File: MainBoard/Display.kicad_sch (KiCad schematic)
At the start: 2 parts, among them CN1 HC-FPC-05-09-22RLTAG, Q2 MMBT2222ALT1G

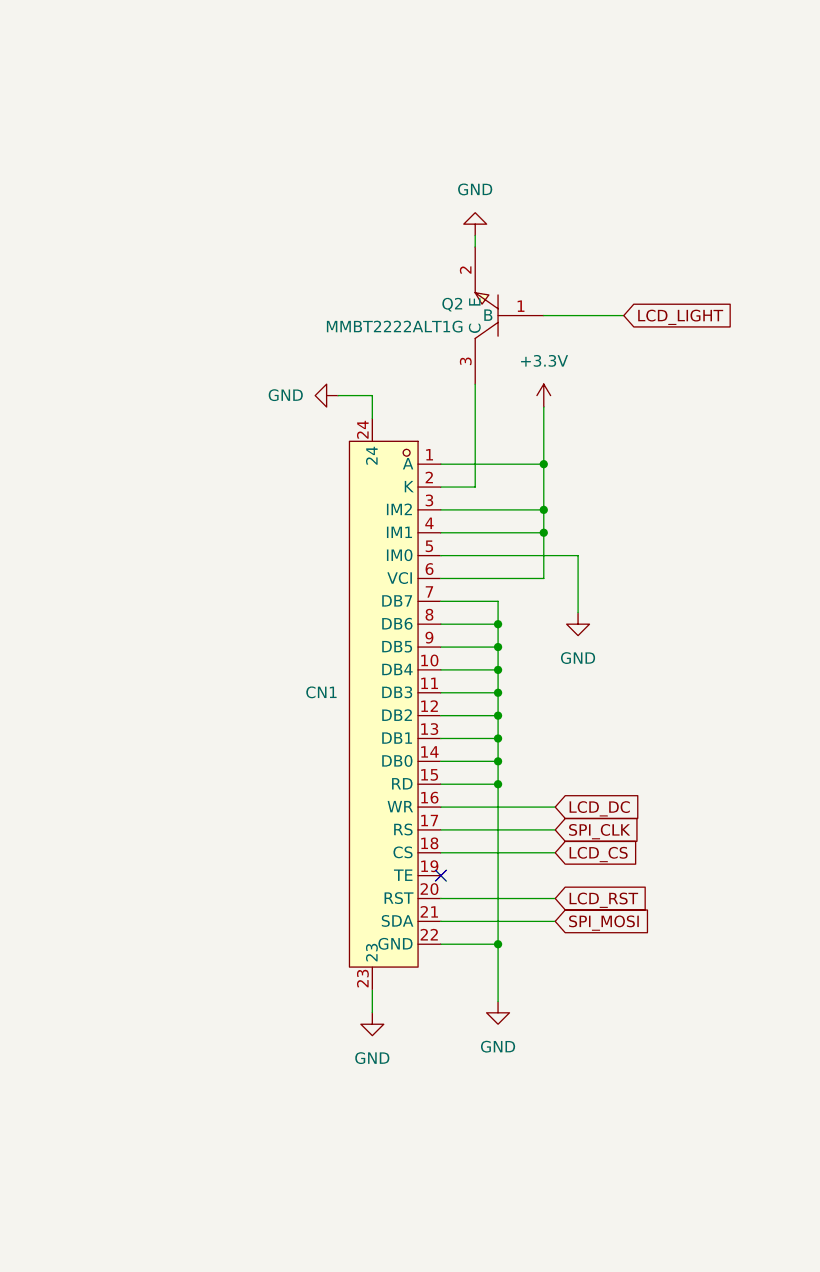
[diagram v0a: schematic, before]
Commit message: layout and starting routing
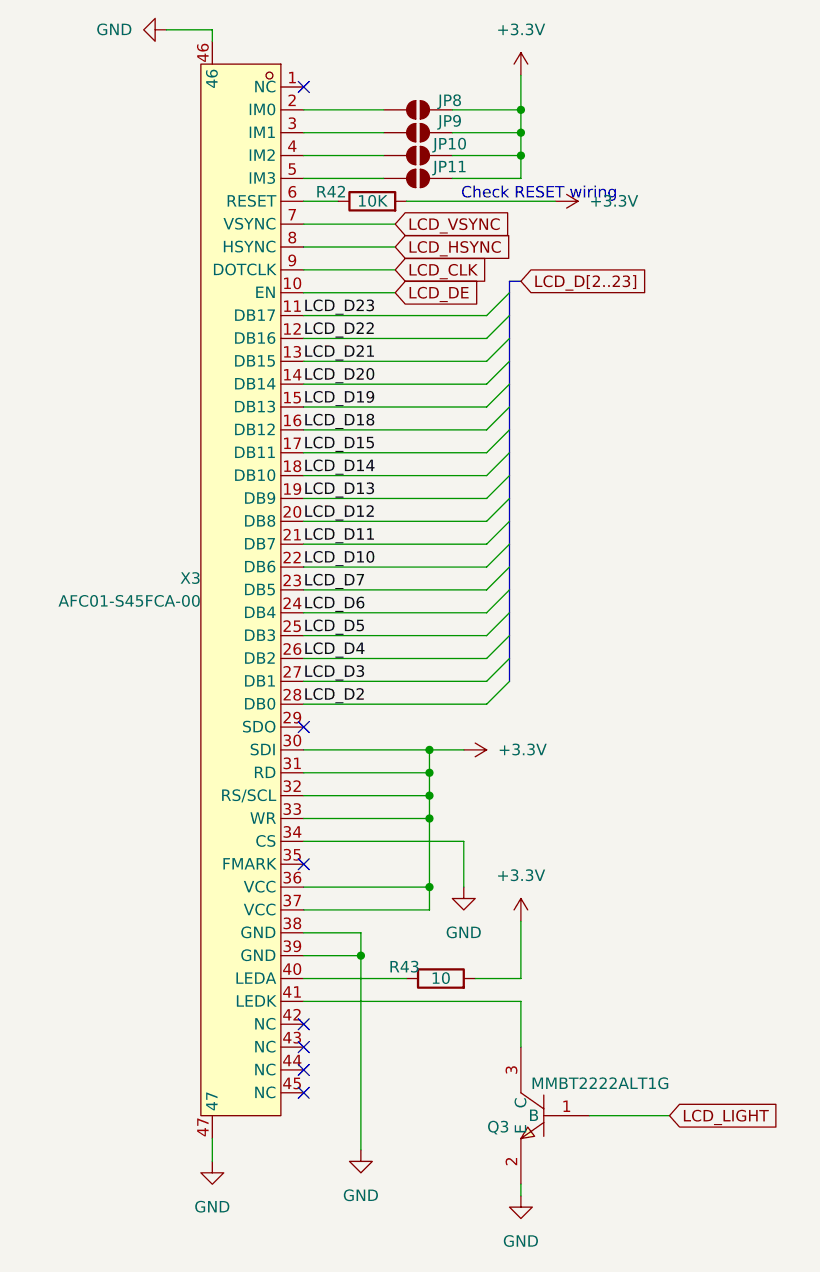
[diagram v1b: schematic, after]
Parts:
- removed CN1: HC-FPC-05-09-22RLTAG, easyeda2kicad:CONN-SMD_22P-P0.50_HCTL_HC-FPC-05-09-22RLTAG, symbol easyeda2kicad:HC-FPC-05-09-22RLTAG
- removed Q2: MMBT2222ALT1G, easyeda2kicad:SOT-23-3_L2.9-W1.3-P1.90-LS2.4-BR, symbol easyeda2kicad:MMBT2222ALT1G
- added JP10, JP11, JP8, JP9: SolderJumper_2_Open, Jumper:SolderJumper-2_P1.3mm_Open_TrianglePad1.0x1.5mm, symbol Jumper:SolderJumper_2_Open
- added Q3: MMBT2222ALT1G, easyeda2kicad:SOT-23-3_L2.9-W1.3-P1.90-LS2.4-BR, symbol easyeda2kicad:MMBT2222ALT1G
- added R42: 10K, Resistor_SMD:R_0402_1005Metric, symbol Device:R
- added R43: 10, Resistor_SMD:R_0402_1005Metric, symbol Device:R
- added X3: AFC01-S45FCA-00, easyeda2kicad:FPC-SMD_AFC01-S45FCA-00, symbol easyeda2kicad:AFC01-S45FCA-00
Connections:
- net +3.3V: now also JP10.2 (B), JP11.2 (B), JP8.2 (B), JP9.2 (B), R42.2, R43.2, X3.30 (SDI), X3.31 (RD), X3.32 (RS/SCL), X3.33 (WR), X3.36 (VCC), X3.37 (VCC)
- net GND: now also Q3.2 (E), X3.34 (CS), X3.38 (GND), X3.39 (GND), X3.46, X3.47
- net LCD_LIGHT: now also Q3.1 (B)
- new net: JP11.1 (A), X3.5 (IM3)
- new net: R42.1, X3.6 (RESET)
- new net: JP10.1 (A), X3.4 (IM2)
- new net: JP8.1 (A), X3.2 (IM0)
- new net: JP9.1 (A), X3.3 (IM1)
- new net: R43.1, X3.40 (LEDA)
- new net: Q3.3 (C), X3.41 (LEDK)
- new net LCD_CLK: X3.9 (DOTCLK)
- new net LCD_D10: X3.22 (DB6)
- new net LCD_D11: X3.21 (DB7)
- new net LCD_D12: X3.20 (DB8)
- new net LCD_D13: X3.19 (DB9)
- new net LCD_D14: X3.18 (DB10)
- new net LCD_D15: X3.17 (DB11)
- new net LCD_D18: X3.16 (DB12)
- new net LCD_D19: X3.15 (DB13)
- new net LCD_D2: X3.28 (DB0)
- new net LCD_D20: X3.14 (DB14)
- new net LCD_D21: X3.13 (DB15)
- new net LCD_D22: X3.12 (DB16)
- new net LCD_D23: X3.11 (DB17)
- new net LCD_D3: X3.27 (DB1)
- new net LCD_D4: X3.26 (DB2)
- new net LCD_D5: X3.25 (DB3)
- new net LCD_D6: X3.24 (DB4)
- new net LCD_D7: X3.23 (DB5)
- new net LCD_DE: X3.10 (EN)
- new net LCD_HSYNC: X3.8 (HSYNC)
- new net LCD_VSYNC: X3.7 (VSYNC)
- no-connect marks 1 -> 7
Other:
- note added: "Check RESET wiring"
